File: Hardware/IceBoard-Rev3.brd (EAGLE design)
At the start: 72.4 x 43.2 mm, 16 parts

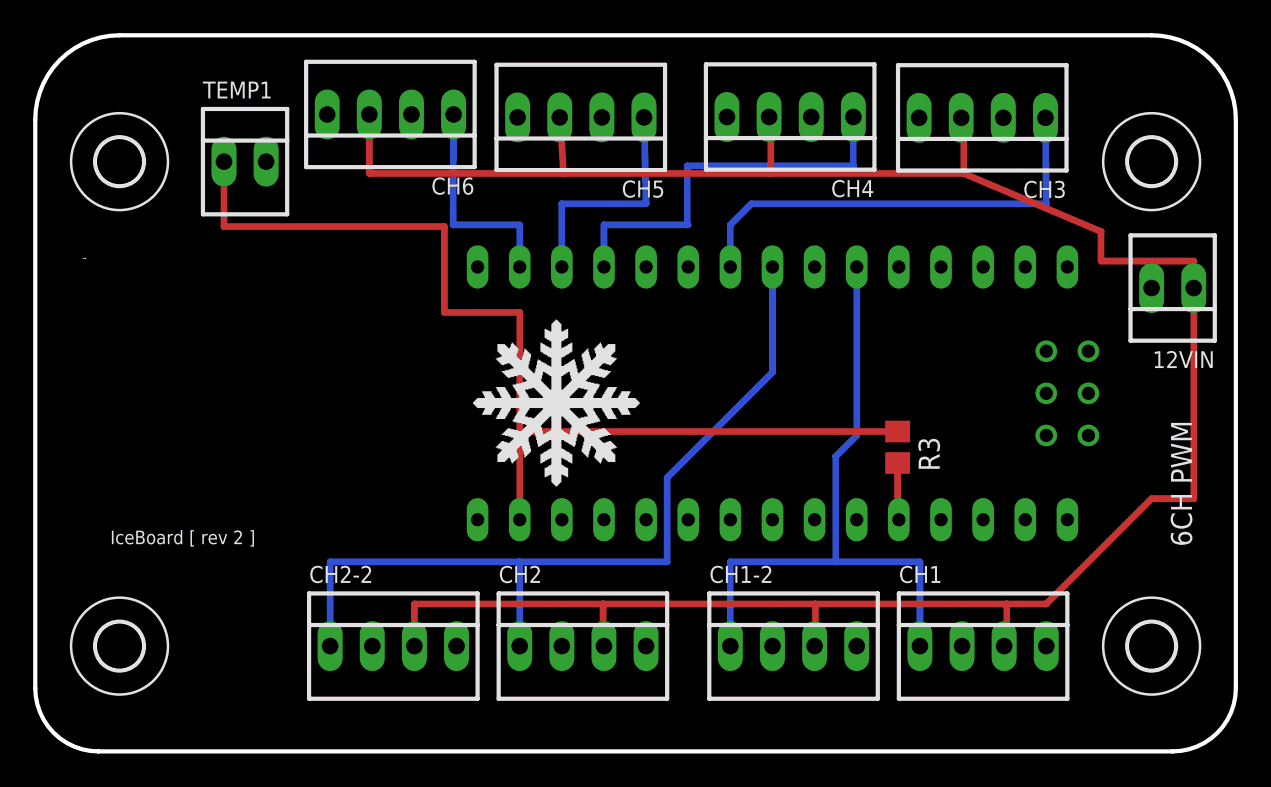
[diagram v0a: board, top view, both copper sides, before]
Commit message: IceBoard Rev3 Hardware
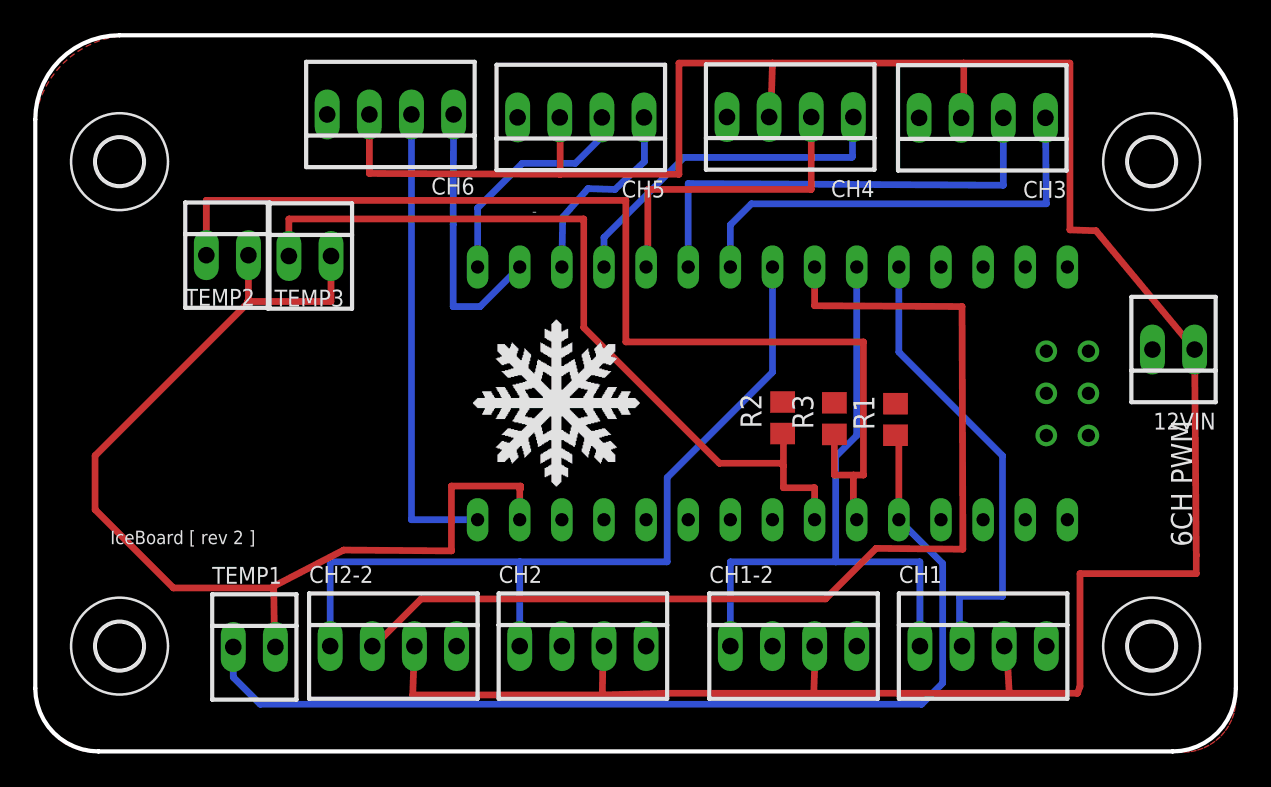
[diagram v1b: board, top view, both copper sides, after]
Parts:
- added R1, R2: 10k, resistor:R0805
- added TEMP2, TEMP3: 22-23-2021, con-molex:22-23-2021
- moved TEMP1 29.3 mm to (27.4, 39.4)
- moved R3 4.18 mm to (62.4, 53.1), turned to 90 degrees
- moved 12VIN 3.71 mm to (82.8, 57.3)
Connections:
- new net N$10: CH5.2, U$1.D12
- new net N$12: CH4.2, U$1.D8
- new net N$13: CH3.2, U$1.D7
- new net N$14: CH2-2.2, U$1.D4
- new net N$15: CH1.2, U$1.D2
- new net N$16: U$1.A2
- new net N$18: R2.1, TEMP3.1, U$1.A5
- new net N$7: R3.1, TEMP2.1, U$1.A6
- new net N$9: CH6.2, U$1.D13
- net 10K: now also TEMP1.2, TEMP2.2, TEMP3.2; no longer R3.1, TEMP1.1
- net GND: now also R1.2, R2.2, R3.2; no longer TEMP1.2
- net N$11: now also R1.1, TEMP1.1; no longer R3.2
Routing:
- net N$7: track 0.00 -> 66.6 mm
- net N$14: track 0.00 -> 63.9 mm
- net N$11: track 3.45 -> 62.0 mm
- net N$18: track 0.00 -> 49.2 mm
- net N$9: track 0.00 -> 28.4 mm
- net N$15: track 0.00 -> 28.1 mm
- net N$13: track 0.00 -> 28.1 mm
- net N$8: track 140.5 -> 163.4 mm
- net N$12: track 0.00 -> 19.0 mm
- net N$10: track 0.00 -> 14.1 mm
- net N$2: track 13.2 -> 16.6 mm
- net N$6: track 24.4 -> 21.4 mm
- net 10K: track 62.2 -> 64.9 mm
- net N$1: track 14.1 -> 12.0 mm
- added copper zone on layer 1, net GND

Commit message: IceBoard Rev3 Hardware
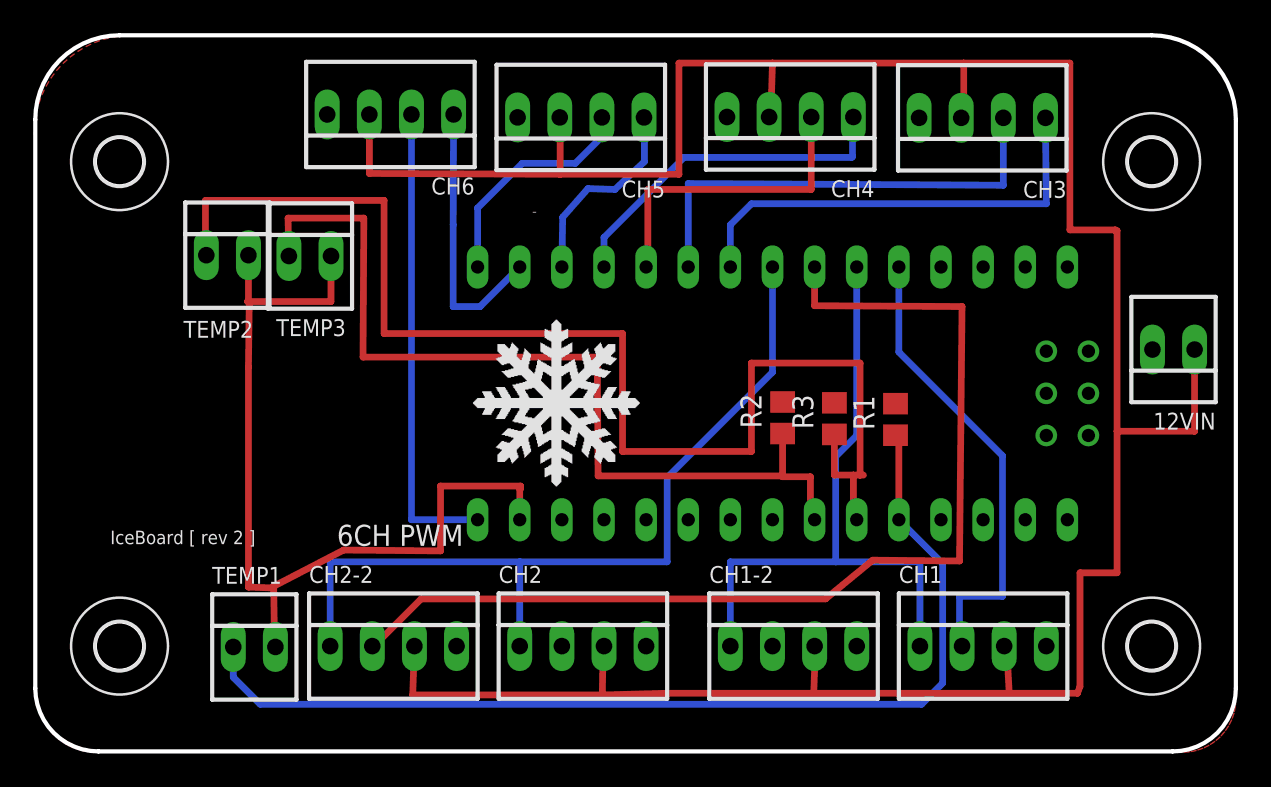
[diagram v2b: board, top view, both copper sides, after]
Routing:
- net N$7: track 66.6 -> 77.2 mm
- net 10K: track 64.9 -> 54.5 mm
- net N$18: track 49.2 -> 54.8 mm
- net N$8: track 163.4 -> 167.4 mm

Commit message: rev3 board
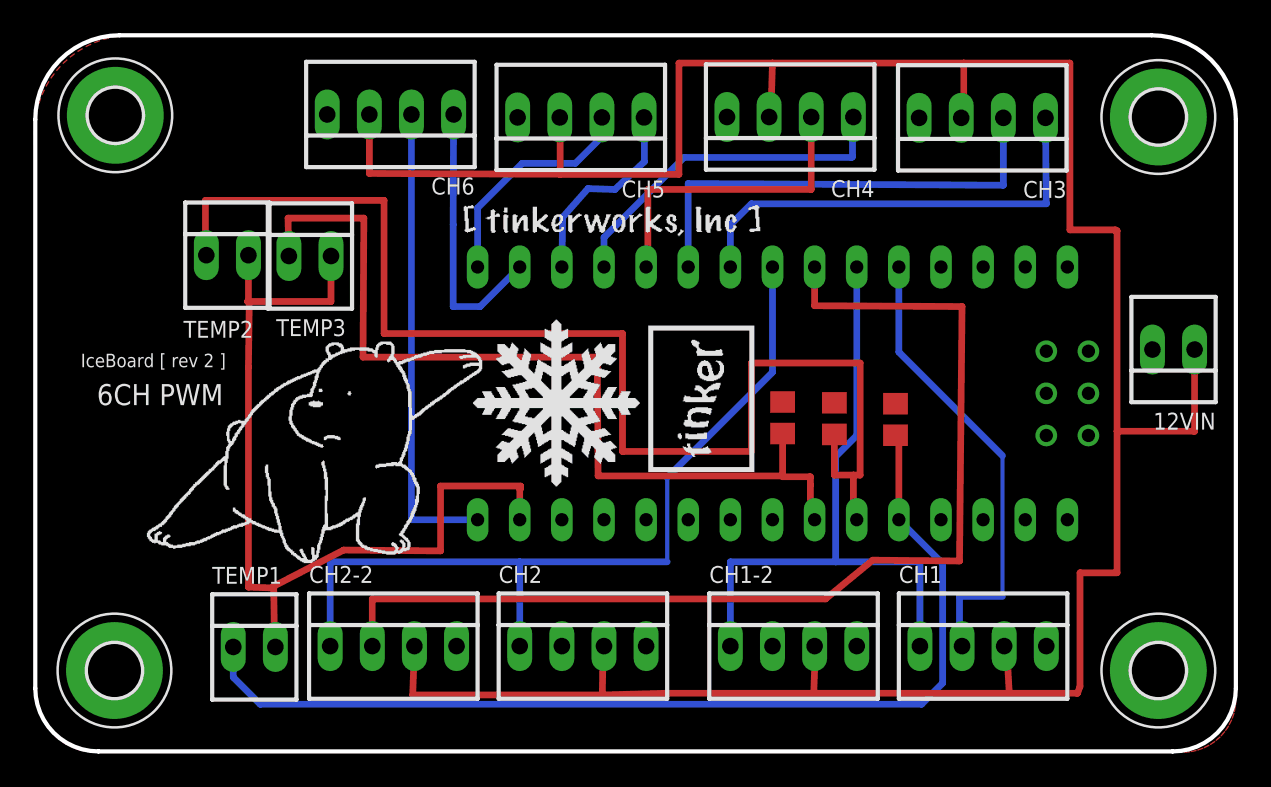
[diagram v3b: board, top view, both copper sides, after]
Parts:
- removed U$2, U$3, U$4, U$5: (no value), holes:2,8
- added H1, H2, H3, H4: MOUNT-PAD-ROUND3.3, holes:3,3-PAD
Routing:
- net N$14: track 64.0 -> 65.8 mm
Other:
- board text removed: "/Users/tink3rbot/Desktop/snowflake.bmp"
- board text removed: "[tink3r]"
